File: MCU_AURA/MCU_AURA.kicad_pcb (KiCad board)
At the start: 4 copper layers, 50 x 50 mm, 82 parts, among them IC1 PCA9685PW,118, J1 TF-CARD_H1.8, J100 USB_C_Receptacle_USB2.0_16P, J200 TC2050-IDC-430, J400 532617004, J401 532617004, J402 532617004, J403 532617010, J404 532617007, J405 532617007, J406 532617012, J407 532614005, Q300 BSS138, Q301 BSS138, Q302 BSS138, U100 TPS2115ADRBR, U101 TLV62566DBVR, U102 AP2127N-1.8, U200 ESP32-S3-WROOM-1, U201 USBLC6-2SC6, U300 ICM-20948, U301 BMP280

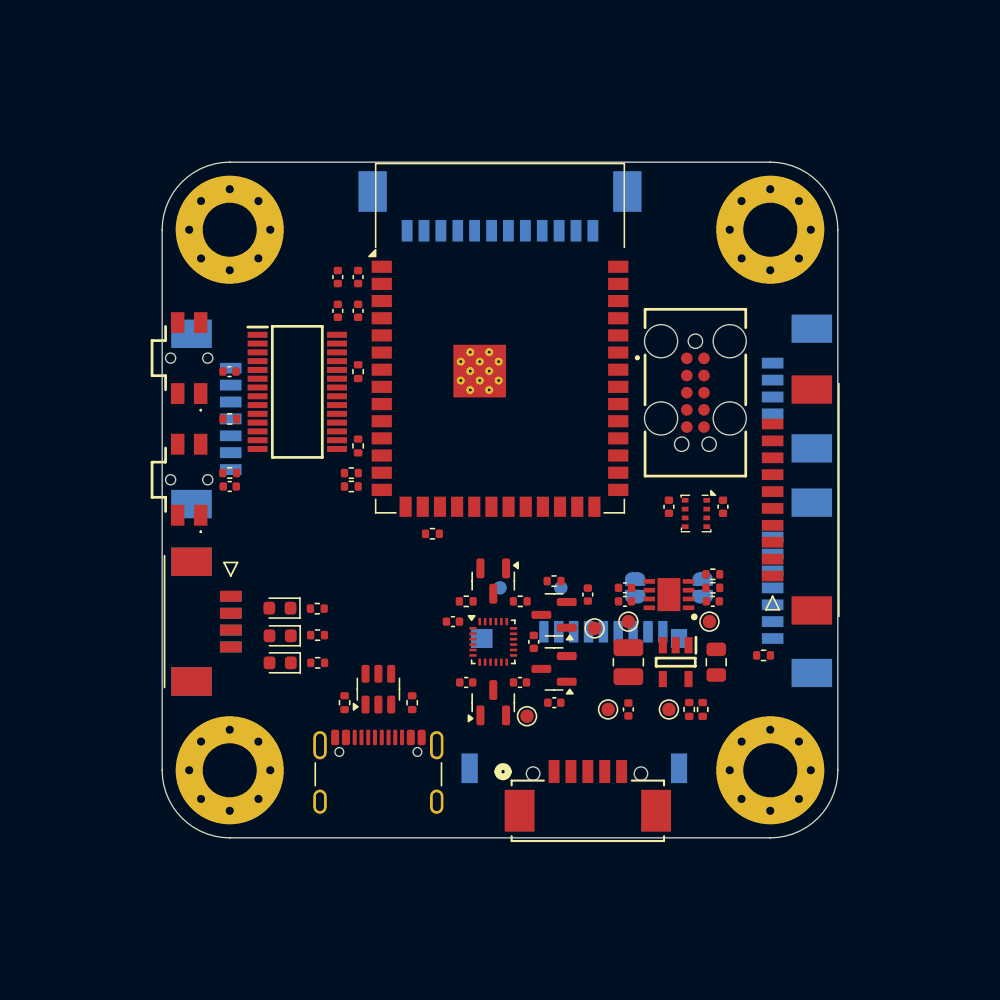
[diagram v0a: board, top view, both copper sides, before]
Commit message: Started Routing
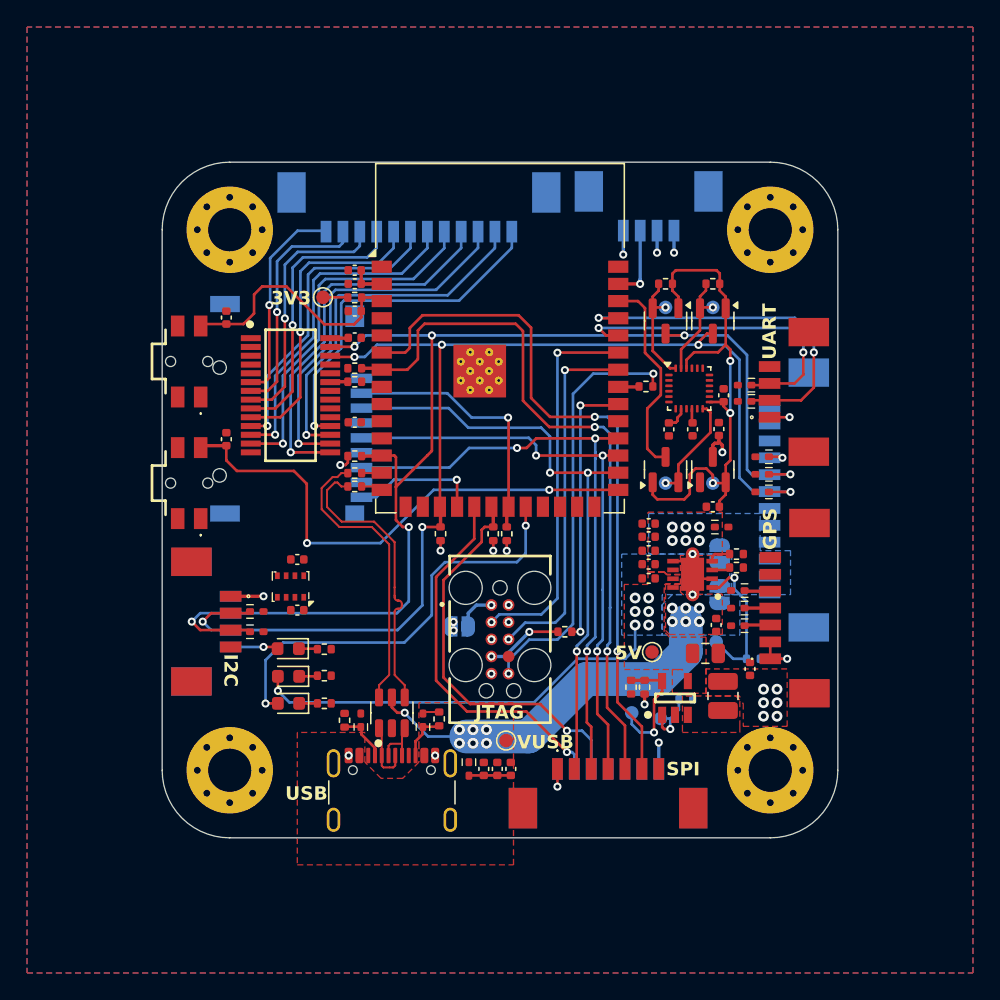
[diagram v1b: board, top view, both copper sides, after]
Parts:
- added C100: 10u, Capacitor_SMD:C_0402_1005Metric, F.Cu at (123.8, 94.9)
- added C101: 1u, Capacitor_SMD:C_0402_1005Metric, F.Cu at (124.8, 94.9)
- added C102: 100n, Capacitor_SMD:C_0402_1005Metric, F.Cu at (125.8, 94.9)
- added C400: 10u, Capacitor_SMD:C_0402_1005Metric, F.Cu at (136.0, 78.8)
- added C401: 1u, Capacitor_SMD:C_0402_1005Metric, F.Cu at (136.0, 77.7)
- added C402: 100n, Capacitor_SMD:C_0402_1005Metric, F.Cu at (136.0, 76.8)
- added D100: TPD1E05U06DPYR, TPD1E05U06DPYR:DIO_TPD1E05U06DPYR, F.Cu at (119.3, 91.3)
- added D101: TPD1E05U06DPYR, TPD1E05U06DPYR:DIO_TPD1E05U06DPYR, F.Cu at (114.7, 91.3)
- added D102: TPD1E05U06DPYR, TPD1E05U06DPYR:DIO_TPD1E05U06DPYR, F.Cu at (122.7, 94.9)
- added D400: TPD1E05U06DPYR, TPD1E05U06DPYR:DIO_TPD1E05U06DPYR, F.Cu at (141.4, 77.0)
- added D401: TPD1E05U06DPYR, TPD1E05U06DPYR:DIO_TPD1E05U06DPYR, F.Cu at (144.4, 71.8)
- added D402: TPD1E05U06DPYR, TPD1E05U06DPYR:DIO_TPD1E05U06DPYR, F.Cu at (144.4, 73.1)
- added D403: TPD1E05U06DPYR, TPD1E05U06DPYR:DIO_TPD1E05U06DPYR, F.Cu at (144.4, 74.4)
- added D404: TPD1E05U06DPYR, TPD1E05U06DPYR:DIO_TPD1E05U06DPYR, F.Cu at (142.6, 84.3)
- added D405: TPD1E05U06DPYR, TPD1E05U06DPYR:DIO_TPD1E05U06DPYR, F.Cu at (142.6, 83.0)
- added D406: TPD1E05U06DPYR, TPD1E05U06DPYR:DIO_TPD1E05U06DPYR, F.Cu at (142.6, 81.7)
- added D407: TPD1E05U06DPYR, TPD1E05U06DPYR:DIO_TPD1E05U06DPYR, F.Cu at (143.1, 67.7)
- added D408: TPD1E05U06DPYR, TPD1E05U06DPYR:DIO_TPD1E05U06DPYR, F.Cu at (143.1, 66.5)
- added D409: TPD1E05U06DPYR, TPD1E05U06DPYR:DIO_TPD1E05U06DPYR, F.Cu at (107.0, 83.2)
- added D410: TPD1E05U06DPYR, TPD1E05U06DPYR:DIO_TPD1E05U06DPYR, F.Cu at (107.0, 84.8)
- added J408: 532617004, 532610471:53261-0471, B.Cu at (136.0, 54.3)
- added JP200: SolderJumper_2_Bridged, Jumper:SolderJumper-2_P1.3mm_Open_RoundedPad1.0x1.5mm, B.Cu at (122.0, 84.4)
- added R1: 22R, Resistor_SMD:R_0402_1005Metric, F.Cu at (129.8, 84.8)
- added R105: 10k, Resistor_SMD:R_0402_1005Metric, B.Cu at (143.8, 86.8)
- added R109: 10k, Resistor_SMD:R_0402_1005Metric, B.Cu at (138.8, 89.8)
- added R2: 22R, Resistor_SMD:R_0402_1005Metric, F.Cu at (135.8, 66.6)
- added TP105: TestPoint, TestPoint:TestPoint_Pad_D1.0mm, B.Cu at (136.9, 91.2)
- H1, H2, H3, H4: footprint MountingHole:MountingHole_4mm_Pad_Via -> MountingHole:MountingHole_3.2mm_M3_Pad_Via
- J400, J401: footprint 532617004:532617004 -> 532610471:53261-0471
- J402: footprint 532617004:532617004 -> 532610471:53261-0471; moved to F.Cu
- J403: value 532617010 -> 532617012; footprint 532617010:532617010 -> 532611271:53261-1271; moved to B.Cu
- J404: footprint 532617007:532617007 -> 532610771:532610771
- J405: footprint 532617007:532617007 -> 532610771:532610771; moved to F.Cu
- J406: footprint 532617012:532617012 -> 532611271:53261-1271
- J407: value 532614005 -> 532617007; footprint 532614005:CONN_532610000-SD_05_MOL -> 532610771:532610771
- R102: value 680R -> 270R
- R103: value 220k -> 10k
- R106: renamed from R105; value 540k -> 68k
- R107: renamed from R106; value 120k -> 15k
- R201, R202: value 27R -> 22R
- TP103, TP302: moved to B.Cu
- TP106: renamed from TP105; moved to B.Cu
- moved J404 39.8 mm to (133.0, 97.4), turned to 0 degrees
- moved TP104 37.1 mm to (111.9, 60.0)
- moved R401 37.0 mm to (114.2, 65.2)
- moved J1 33.1 mm to (107.5, 68.2), turned to 90 degrees
- moved U301 30.5 mm to (109.5, 81.4), turned to 180 degrees
- moved C201 28.5 mm to (114.2, 59.0), turned to 180 degrees
- moved C306 28.0 mm to (114.2, 69.2), turned to 180 degrees
- moved R300 27.7 mm to (137.2, 59.0), turned to 0 degrees
- moved R301 27.5 mm to (140.8, 59.0), turned to 0 degrees
- moved C301 26.1 mm to (141.6, 67.2), turned to 90 degrees
- moved Q301 24.7 mm to (140.8, 61.8), turned to -90 degrees
- moved TP300 24.1 mm to (137.2, 60.8)
- moved C300 24.0 mm to (137.5, 69.8), turned to -90 degrees
- moved U300 23.7 mm to (139.0, 66.8)
- moved C108 23.6 mm to (141.2, 69.8), turned to 90 degrees
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- renumbered C100 to C103, C101 to C104, C102 to C105, C103 to C106, C104 to C107, C105 to C108, C106 to C109, D100 to D103, D103 to D104, R107 to R108
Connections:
- net /100_Power/ILIM_5V_SW renamed /100_Power/ILIM_5V
- net Net-(IC1-~{OE}) renamed /300_Digital_Peripherals/MUX_OE
- C203 pad 1: /200_ESP32/RST -> /200_ESP32/EN
- C204 pad 1: /200_ESP32/EN -> /200_ESP32/RST
- J200 pad 1: +3V3 -> /200_ESP32/JTAG_3V3
- J403 pad 1: +5V -> GND
- J403 pad 10: GND -> +5V
- J403 pad 11: (no net) -> +5V
- J403 pad 12: (no net) -> +5V
- J403 pad 2: +5V -> GND
- J403 pad 3: +3V3 -> GND
- J403 pad 4: SCL -> +3V3
- J403 pad 6: GND -> SCL
- J403 pad 7: MSFT_1 -> GND
- J403 pad 8: MSFT_2 -> MSFT_1
- J403 pad 9: GND -> MSFT_2
- J407 pad 2: GPS_TX -> +3V3
- J407 pad 3: GPS_RX -> GPS_TX
- J407 pad 4: GPS_INT -> GPS_RX
- J407 pad 5: GND -> GPS_INT
- J407 pad 6: (no net) -> GND
- J407 pad 7: (no net) -> GND
- R100 pad 2: /100_Power/CC1 -> /100_Power/CC2
- R101 pad 2: /100_Power/CC2 -> /100_Power/CC1
- S200 pad 2: /200_ESP32/RST -> GND
- S200 pad 3: GND -> /200_ESP32/EN
- S201 pad 2: /200_ESP32/EN -> GND
- S201 pad 3: GND -> /200_ESP32/RST
- U101 pad 1: +5V_FILT -> /100_Power/PG_3V3
- U200 pad 32: /200_ESP32/TCK -> /200_ESP32/TCK_D
- U200 pad 33: /200_ESP32/TDO -> /200_ESP32/TDO_D
- U200 pad 38: unconnected-(U200-IO2-Pad38) -> ICM_INT
- U200 pad 39: unconnected-(U200-IO1-Pad39) -> RC_RX
- U200 pad 8: ICM_INT -> unconnected-(U200-IO15-Pad8)
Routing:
- net SDA: track 0.00 -> 94.3 mm, vias 0 -> 6
- net SCL: track 0.00 -> 90.7 mm, vias 0 -> 6
- net EXT_CS: track 0.00 -> 52.9 mm, vias 0 -> 2
- net EXT_RST: track 0.00 -> 52.0 mm, vias 0 -> 2
- net MISO: track 0.00 -> 45.0 mm, vias 0 -> 3
- net MOSI: track 0.00 -> 44.9 mm, vias 0 -> 3
- net SCK: track 0.00 -> 43.9 mm, vias 0 -> 3
- net +1V8: track 0.00 -> 41.2 mm, vias 0 -> 3
- net /200_ESP32/RST: track 0.00 -> 38.8 mm, vias 0 -> 2
- net +3V3: track 0.00 -> 32.1 mm, vias 0 -> 22
- net LED: track 0.00 -> 31.8 mm, vias 0 -> 2
- net /200_ESP32/TDO: track 0.00 -> 31.7 mm, vias 0 -> 2
- net +5V_FILT: track 0.00 -> 31.3 mm, vias 0 -> 7
- net +VUSB: track 0.00 -> 29.6 mm, vias 0 -> 13
- net RF_CS: track 0.00 -> 29.6 mm, vias 0 -> 1
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- added copper zone on F.Cu, net +3V3
- added copper zone on In1.Cu, net +3V3
- added copper zone on In2.Cu, net +3V3
- added copper zone on B.Cu, net +5V
- added copper zone on F.Cu, net +5V
- added copper zone on B.Cu, net +5V_FILT
- added copper zone on F.Cu, net +5V_FILT
- added copper zone on B.Cu, net +VUSB
- added copper zone on F.Cu, net +VUSB
- added copper zone on F.Cu, net /100_Power/SW_3V3
- added copper zone on B.Cu, net GND
- added copper zone on F.Cu, net GND
- added copper zone on In1.Cu, net GND
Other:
- board text added: "1V8"
- board text added: "3V3"
- board text added: "5V"
- board text added: "FB"
- board text added: "GPS"
- board text added: "I2C"
- board text added: "INT"
- board text added: "JTAG"
- board text added: "PG"
- board text added: "POWER"
- board text added: "RADIO"
- board text added: "SCL"
- board text added: "SD"
- board text added: "SDA"
- board text added: "SERVOS"
- board text added: "SPI"
- board text added: "STAT"
- board text added: "UART"
- board text added: "USB"
- board text added: "VUSB"
